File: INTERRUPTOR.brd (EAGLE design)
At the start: 39.8 x 21.5 mm, 6 parts, among them J1 CONECTOR_MACHO, J2 CONECTOR_FEMEA, J3 SS12F46, U1 74HC132

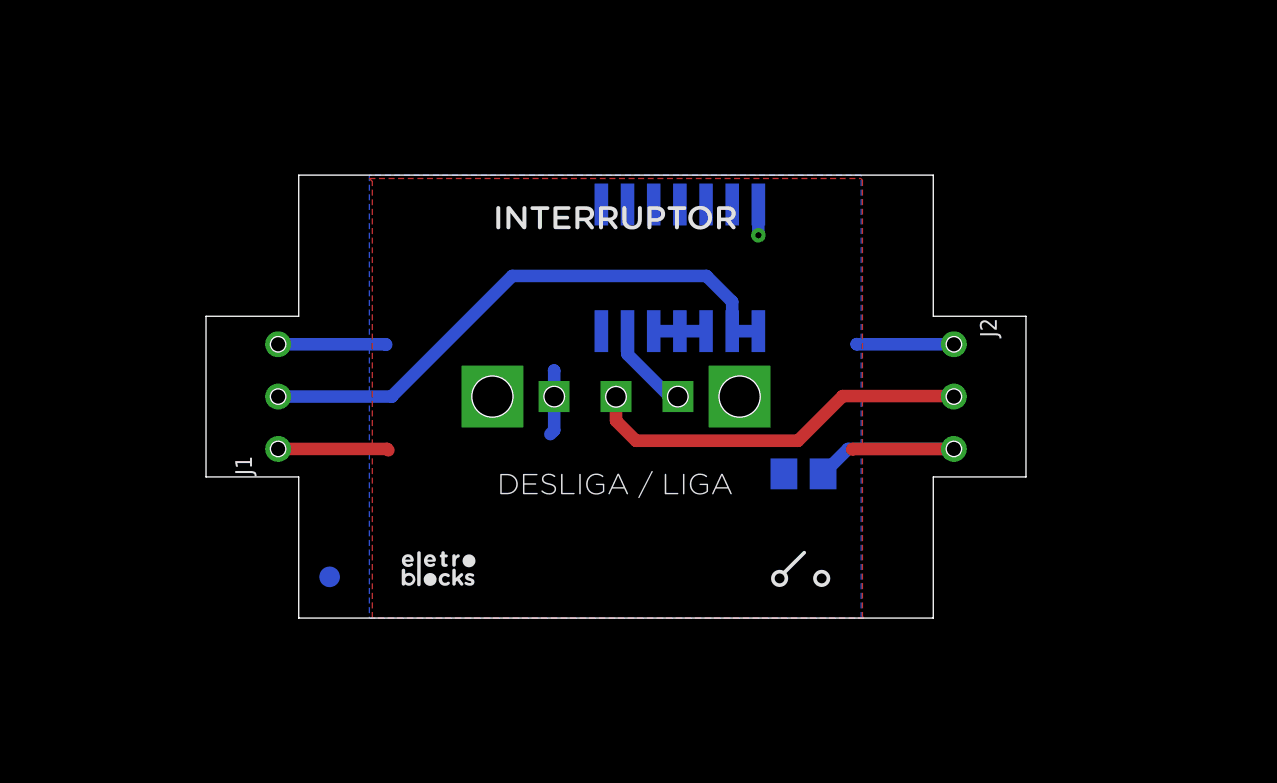
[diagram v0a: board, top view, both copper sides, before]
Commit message: V1.0.2
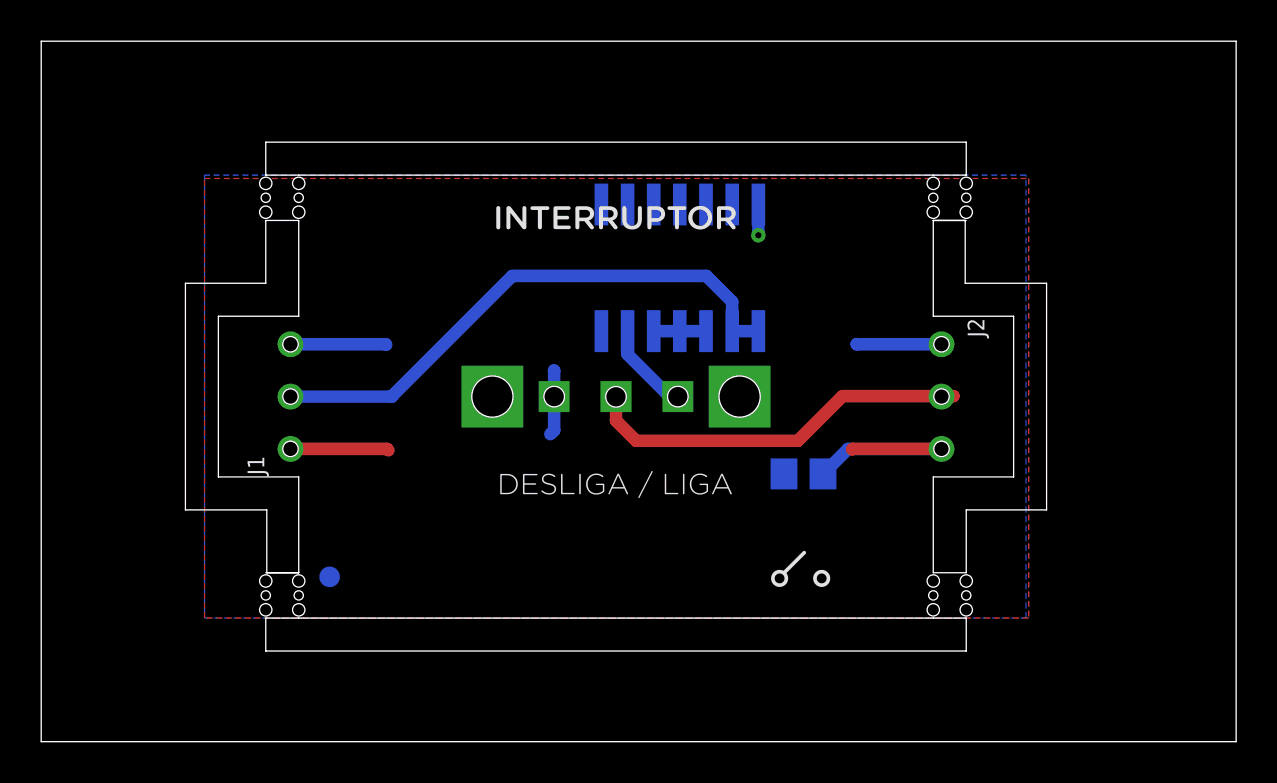
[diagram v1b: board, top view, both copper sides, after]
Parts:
- added U$1, U$3, U$4, U$5: (no value), Eletroblocks Lib:STAMP_DUPLO
- J1: device Eletroblocks Lib:3CONECTOR -> Eletroblocks Lib:MALE
- J2: device Eletroblocks Lib:3CONECTOR -> Eletroblocks Lib:FEMALE
- moved J2 0.60 mm to (27.7, 10.8)
- moved J1 0.60 mm to (-3.90, 10.8)
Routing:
- net VCC: track 18.7 -> 16.9 mm
- net GND: track 13.2 -> 12.0 mm
- net SIGNAL_IN: track 27.7 -> 27.1 mm
- net SIGNAL_OUT: track 18.9 -> 19.4 mm
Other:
- board size 39.8 x 21.5 mm -> 58 x 34 mm
- board text added: "V1.0.2"
- board text removed: "V1.0.1"
